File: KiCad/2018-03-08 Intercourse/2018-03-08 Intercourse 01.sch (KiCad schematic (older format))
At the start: 18 parts

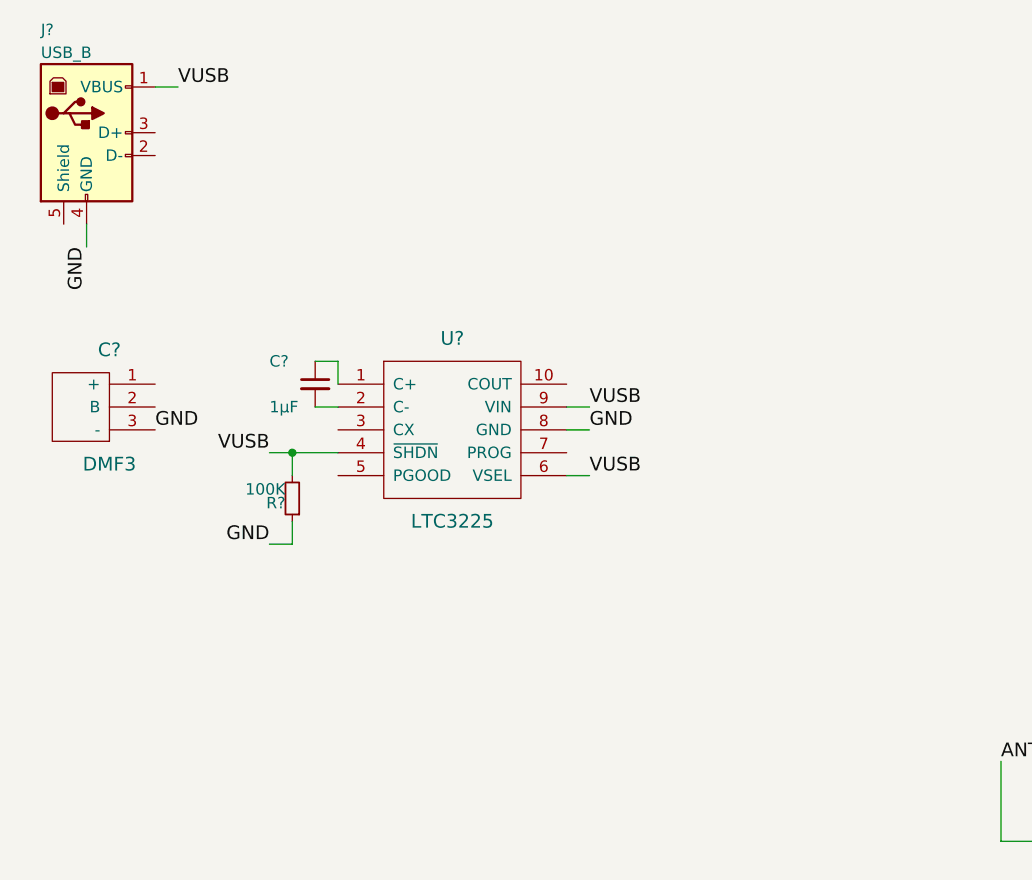
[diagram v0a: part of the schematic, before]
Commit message: charge pump done
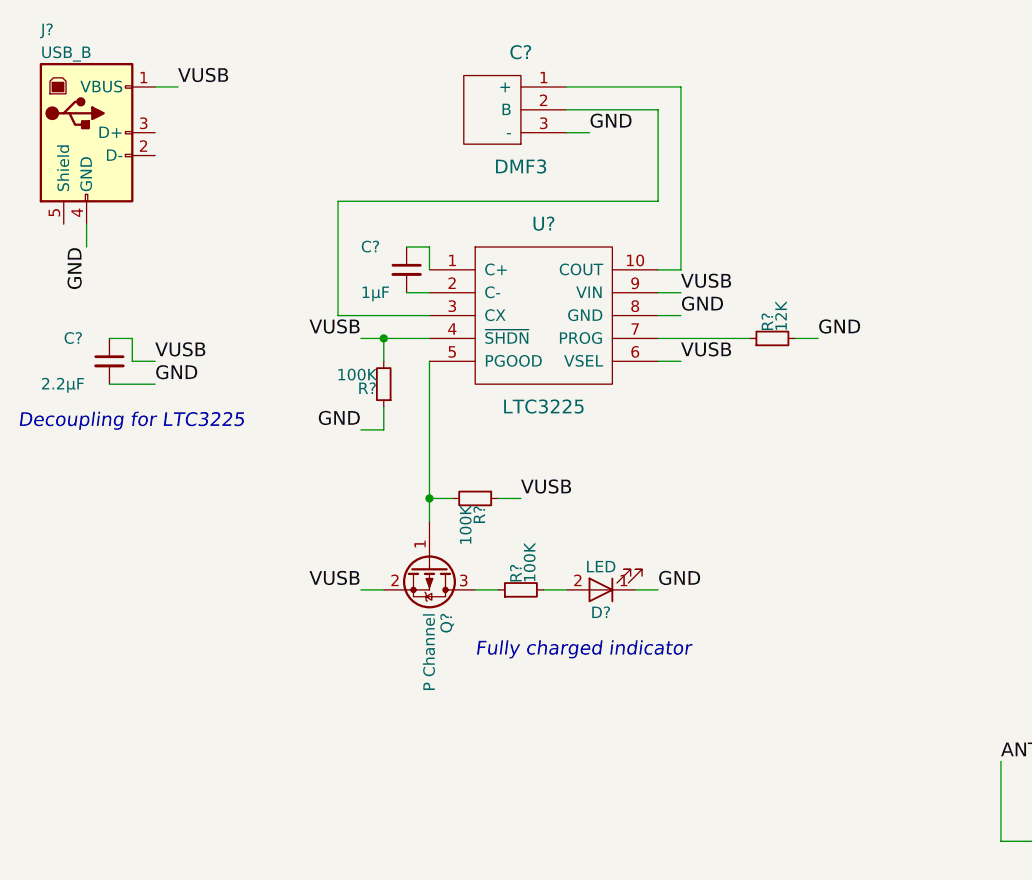
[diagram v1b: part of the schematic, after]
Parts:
- added C?: 2.2μF, symbol C_Small
- added D?: LED, symbol LED
- added Q?: P Channel, TO_SOT_Packages_SMD:SOT-23, symbol TP0610T
- added R?: 12K, symbol R_Small
- added R? (x2): 100K, symbol R_Small
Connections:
- net GND: now also C?.2, D?.1 (K), R?.2
- net VUSB: now also C?.1, Q?.2 (S), R?.1
- net at C?.1 (+): now also U?.10 (COUT)
- net at C?.2 (B): now also U?.3 (CX)
- net at U?.5 (PGOOD): now also Q?.1 (G), R?.2
- net at U?.7 (PROG): now also R?.1
- new net: Q?.3 (D), R?.1
- new net: D?.2 (A), R?.2
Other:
- note added: "Decoupling for LTC3225"
- note added: "Fully charged indicator"
- moved on the sheet: C?, R?, U?
